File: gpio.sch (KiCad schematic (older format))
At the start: 3 parts, among them J1 DF40C-100DP-0.4V(51), J2 DF40C-100DP-0.4V(51), U1 LFE5U-85F-6BG381C

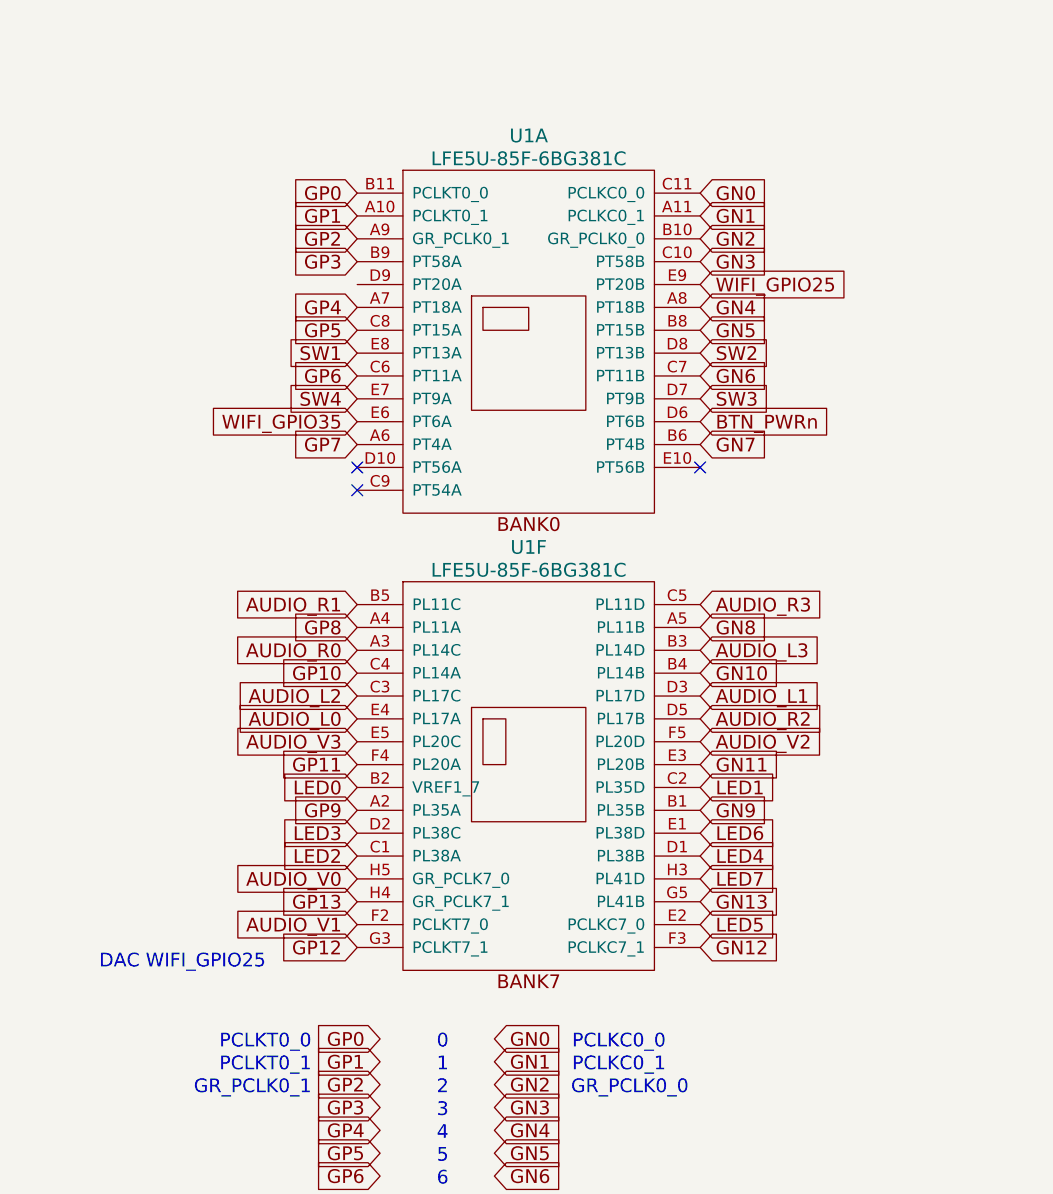
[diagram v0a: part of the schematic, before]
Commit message: Adding connectors
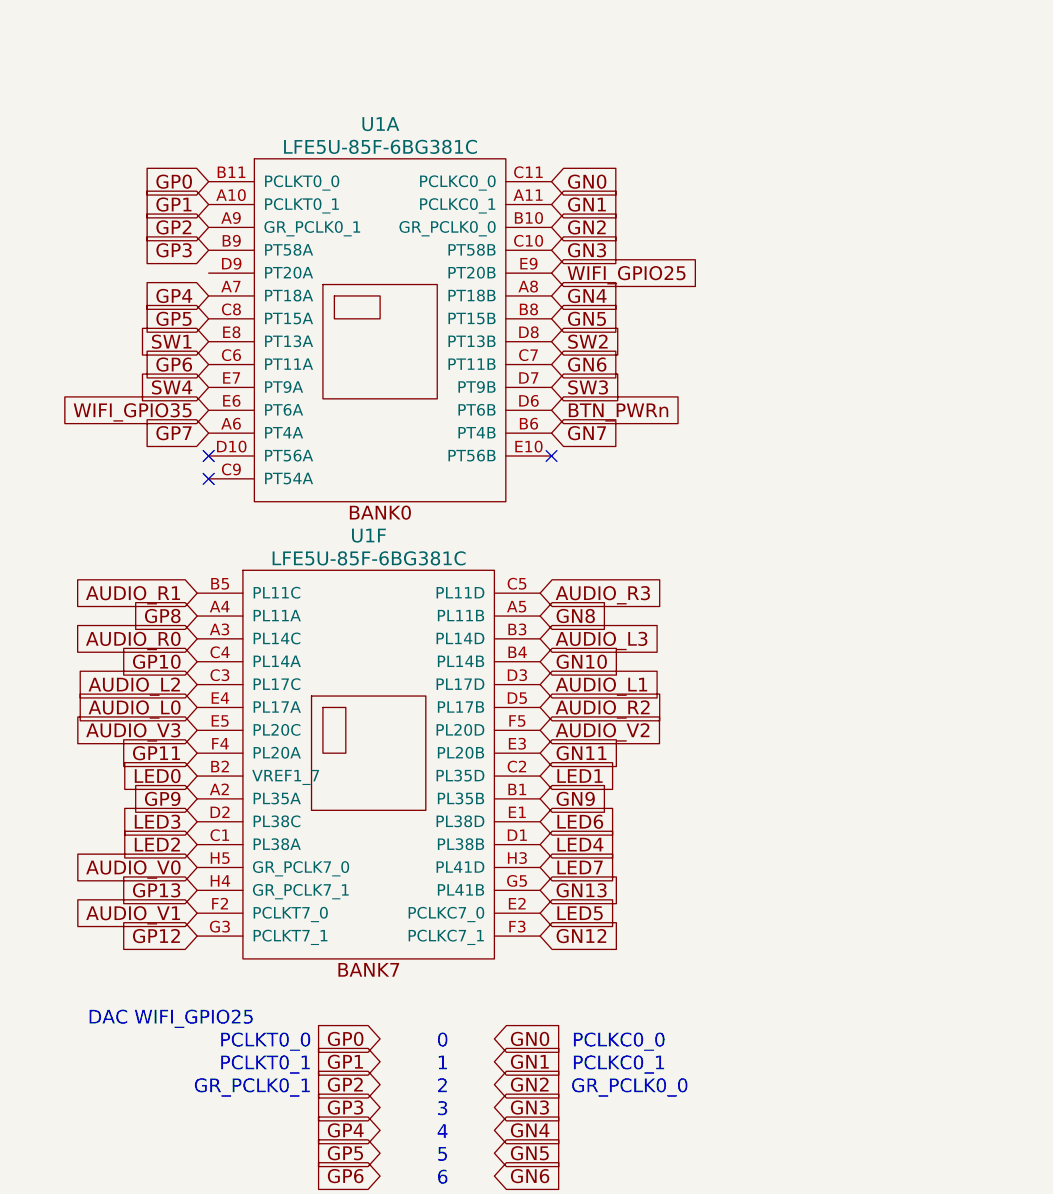
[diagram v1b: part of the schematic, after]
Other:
- moved on the sheet: U1A, U1F
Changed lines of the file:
@@
 Text GLabel 5350 6200 2    60   Input ~ 0
 GP27
-Text GLabel 3250 3950 2    60   Input ~ 0
+Text GLabel 2550 3900 2    60   Input ~ 0
 GN13
-Text GLabel 1750 3950 0    60   Input ~ 0
+Text GLabel 1050 3900 0    60   Input ~ 0
 GP13
-Text GLabel 1750 4150 0    60   Input ~ 0
+Text GLabel 1050 4100 0    60   Input ~ 0
 GP12
-Text GLabel 3250 4150 2    60   Input ~ 0
+Text GLabel 2550 4100 2    60   Input ~ 0
 GN12
-Text GLabel 3250 3350 2    60   Input ~ 0
+Text GLabel 2550 3300 2    60   Input ~ 0
 GN11
-Text GLabel 1750 3350 0    60   Input ~ 0
+Text GLabel 1050 3300 0    60   Input ~ 0
 GP11
-Text GLabel 3250 3550 2    60   Input ~ 0
+Text GLabel 2550 3500 2    60   Input ~ 0
 GN9
-Text GLabel 1750 3550 0    60   Input ~ 0
+Text GLabel 1050 3500 0    60   Input ~ 0
 GP9
-Text GLabel 3250 2950 2    60   Input ~ 0
+Text GLabel 2550 2900 2    60   Input ~ 0
 GN10
-Text GLabel 1750 2950 0    60   Input ~ 0
+Text GLabel 1050 2900 0    60   Input ~ 0
 GP10
-Text GLabel 3250 2750 2    60   Input ~ 0
+Text GLabel 2550 2700 2    60   Input ~ 0
 GN8
-Text GLabel 1750 2750 0    60   Input ~ 0
+Text GLabel 1050 2700 0    60   Input ~ 0
 GP8
-Text GLabel 3250 1950 2    60   Input ~ 0
+Text GLabel 2600 1900 2    60   Input ~ 0
 GN7
-Text GLabel 1750 1950 0    60   Input ~ 0
+Text GLabel 1100 1900 0    60   Input ~ 0
 GP7
-Text GLabel 3250 1650 2    60   Input ~ 0
+Text GLabel 2600 1600 2    60   Input ~ 0
 GN6
-Text GLabel 1750 1650 0    60   Input ~ 0
+Text GLabel 1100 1600 0    60   Input ~ 0
 GP6
-Text GLabel 3250 850  2    60   Input ~ 0
+Text GLabel 2600 800  2    60   Input ~ 0
 GN0
-Text GLabel 3250 950  2    60   Input ~ 0
+Text GLabel 2600 900  2    60   Input ~ 0
 GN1
-Text GLabel 3250 1050 2    60   Input ~ 0
+Text GLabel 2600 1000 2    60   Input ~ 0
 GN2
-Text GLabel 3250 1350 2    60   Input ~ 0
+Text GLabel 2600 1300 2    60   Input ~ 0
 GN4
-Text GLabel 1750 850  0    60   Input ~ 0
+Text GLabel 1100 800  0    60   Input ~ 0
 GP0
-Text GLabel 1750 950  0    60   Input ~ 0
+Text GLabel 1100 900  0    60   Input ~ 0
 GP1
-Text GLabel 1750 1050 0    60   Input ~ 0
+Text GLabel 1100 1000 0    60   Input ~ 0
 GP2
-Text GLabel 1750 1350 0    60   Input ~ 0
+Text GLabel 1100 1300 0    60   Input ~ 0
 GP4
-Text GLabel 1750 1450 0    60   Input ~ 0
+Text GLabel 1100 1400 0    60   Input ~ 0
 GP5
-Text GLabel 3250 1450 2    60   Input ~ 0
+Text GLabel 2600 1400 2    60   Input ~ 0
 GN5
-Text GLabel 3250 1150 2    60   Input ~ 0
+Text GLabel 2600 1100 2    60   Input ~ 0
 GN3
-Text GLabel 1750 1150 0    60   Input ~ 0
+Text GLabel 1100 1100 0    60   Input ~ 0
 GP3
-Text GLabel 1750 3150 0    60   Input ~ 0
+Text GLabel 1050 3100 0    60   Input ~ 0
 AUDIO_L0
-Text GLabel 3250 3050 2    60   Input ~ 0
+Text GLabel 2550 3000 2    60   Input ~ 0
 AUDIO_L1
-Text GLabel 1750 3050 0    60   Input ~ 0
+Text GLabel 1050 3000 0    60   Input ~ 0
 AUDIO_L2
-Text GLabel 3250 2850 2    60   Input ~ 0
+Text GLabel 2550 2800 2    60   Input ~ 0
 AUDIO_L3
-Text GLabel 1750 2850 0    60   Input ~ 0
+Text GLabel 1050 2800 0    60   Input ~ 0
 AUDIO_R0
-Text GLabel 1750 2650 0    60   Input ~ 0
+Text GLabel 1050 2600 0    60   Input ~ 0
 AUDIO_R1
-Text GLabel 3250 3150 2    60   Input ~ 0
+Text GLabel 2550 3100 2    60   Input ~ 0
 AUDIO_R2
-Text GLabel 3250 2650 2    60   Input ~ 0
+Text GLabel 2550 2600 2    60   Input ~ 0
 AUDIO_R3
-Text GLabel 1750 3450 0    60   Input ~ 0
+Text GLabel 1050 3400 0    60   Input ~ 0
 LED0
-Text GLabel 3250 4050 2    60   Input ~ 0
+Text GLabel 2550 4000 2    60   Input ~ 0
 LED5
-Text GLabel 1750 3750 0    60   Input ~ 0
+Text GLabel 1050 3700 0    60   Input ~ 0
 LED2
-Text GLabel 1750 3650 0    60   Input ~ 0
+Text GLabel 1050 3600 0    60   Input ~ 0
 LED3
-Text GLabel 3250 3750 2    60   Input ~ 0
+Text GLabel 2550 3700 2    60   Input ~ 0
 LED4
-Text GLabel 3250 3450 2    60   Input ~ 0
+Text GLabel 2550 3400 2    60   Input ~ 0
 LED1
-Text GLabel 3250 3650 2    60   Input ~ 0
+Text GLabel 2550 3600 2    60   Input ~ 0
 LED6
-Text GLabel 3250 3850 2    60   Input ~ 0
+Text GLabel 2550 3800 2    60   Input ~ 0
 LED7
 Text Notes 950  7550 0    60   ~ 0
 GPIO route only A/B pairs as those are differential bidirectional\ndon't route C/D pairs to GPIO as those can be differential input only\nBANK0,1 are single-ended (non-differential)
-Text GLabel 3250 1850 2    60   Input ~ 0
+Text GLabel 2600 1800 2    60   Input ~ 0
 BTN_PWRn
 Text Notes 950  7200 0    60   ~ 0
 GP,GN 14-21 differential bidirectional connected to BANK2,3 on "ram" sheet\nGP,GN 22-27 single-ended connected to BANK1 on "gpdi" sheet
-Text GLabel 1750 1550 0    60   Input ~ 0
+Text GLabel 1100 1500 0    60   Input ~ 0
 SW1
-Text GLabel 3250 1550 2    60   Input ~ 0
+Text GLabel 2600 1500 2    60   Input ~ 0
 SW2
-Text GLabel 3250 1750 2    60   Input ~ 0
+Text GLabel 2600 1700 2    60   Input ~ 0
 SW3
-Text GLabel 1750 1750 0    60   Input ~ 0
+Text GLabel 1100 1700 0    60   Input ~ 0
 SW4
-Text GLabel 1750 3250 0    60   Input ~ 0
+Text GLabel 1050 3200 0    60   Input ~ 0
 AUDIO_V3
-Text GLabel 3250 3250 2    60   Input ~ 0
+Text GLabel 2550 3200 2    60   Input ~ 0
 AUDIO_V2
-Text GLabel 1750 4050 0    60   Input ~ 0
+Text GLabel 1050 4000 0    60   Input ~ 0
 AUDIO_V1
-Text GLabel 1750 3850 0    60   Input ~ 0
+Text GLabel 1050 3800 0    60   Input ~ 0
 AUDIO_V0
 $Comp
 L lfe5bg381:LFE5UM-85F-6BG381C U1
 U 6 1 5A0783C9
-P 2500 3350
+P 1800 3300
 AR Path="/5A0783C9" Ref="U1"  Part="6"
 AR Path="/56AC389C/5A0783C9" Ref="U1"  Part="6"
-F 0 "U1" H 2500 4300 60  0000 C CNN
-F 1 "LFE5U-85F-6BG381C" H 2500 4200 60  0000 C CNN
-F 2 "lfe5bg381:BGA-381_pitch0.8mm_dia0.4mm" H 1450 4300 60  0001 C CNN
-F 3 "http://www.latticesemi.com/~/media/LatticeSemi/Documents/DataSheets/ECP5/FPGA-DS-02012.pdf" H 1450 4300 60  0001 C CNN
-F 4 "LFE5U-85F-6BG381C" H 2500 3350 60  0001 C CNN "MPN"
-	6    2500 3350
+F 0 "U1" H 1800 4250 60  0000 C CNN
+F 1 "LFE5U-85F-6BG381C" H 1800 4150 60  0000 C CNN
+F 2 "lfe5bg381:BGA-381_pitch0.8mm_dia0.4mm" H 750 4250 60  0001 C CNN
+F 3 "http://www.latticesemi.com/~/media/LatticeSemi/Documents/DataSheets/ECP5/FPGA-DS-02012.pdf" H 750 4250 60  0001 C CNN
+F 4 "LFE5U-85F-6BG381C" H 1800 3300 60  0001 C CNN "MPN"
+	6    1800 3300
 	1    0    0    -1
 $EndComp
@@
 L lfe5bg381:LFE5UM-85F-6BG381C U1
 U 1 1 5A0737C6
-P 2500 1550
+P 1850 1500
 AR Path="/5A0737C6" Ref="U1"  Part="1"
 AR Path="/56AC389C/5A0737C6" Ref="U1"  Part="1"
-F 0 "U1" H 2500 2500 60  0000 C CNN
-F 1 "LFE5U-85F-6BG381C" H 2500 2400 60  0000 C CNN
-F 2 "lfe5bg381:BGA-381_pitch0.8mm_dia0.4mm" H 1450 2500 60  0001 C CNN
-F 3 "http://www.latticesemi.com/~/media/LatticeSemi/Documents/DataSheets/ECP5/FPGA-DS-02012.pdf" H 1450 2500 60  0001 C CNN
-F 4 "LFE5U-85F-6BG381C" H 2500 1550 60  0001 C CNN "MPN"
-	1    2500 1550
+F 0 "U1" H 1850 2450 60  0000 C CNN
+F 1 "LFE5U-85F-6BG381C" H 1850 2350 60  0000 C CNN
+F 2 "lfe5bg381:BGA-381_pitch0.8mm_dia0.4mm" H 800 2450 60  0001 C CNN
+F 3 "http://www.latticesemi.com/~/media/LatticeSemi/Documents/DataSheets/ECP5/FPGA-DS-02012.pdf" H 800 2450 60  0001 C CNN
+F 4 "LFE5U-85F-6BG381C" H 1850 1500 60  0001 C CNN "MPN"
+	1    1850 1500
 	1    0    0    -1
 $EndComp
@@
 Text Notes 6300 7150 0    60   ~ 0
 STPS2L40AF
-NoConn ~ 1750 2050
-NoConn ~ 1750 2150
-NoConn ~ 3250 2050
+NoConn ~ 1100 2000
+NoConn ~ 1100 2100
+NoConn ~ 2600 2000
 Text Notes 1500 6100 2    60   ~ 0
 GR_PCLK7_1
@@
 Text Notes 3200 4800 2    60   ~ 0
 GR_PCLK0_0
-Text Notes 1350 4250 2    60   ~ 0
+Text Notes 1300 4500 2    60   ~ 0
 DAC WIFI_GPIO25
 Text Notes 1500 5900 2    60   ~ 0
@@
 Text Notes 950  6450 0    60   ~ 0
 J1 J2 PIN numbering 1-40 is for FEMALE 90° ANGLED header.\nFor MALE VERTICAL header, SWAP EVEN and ODD pin numbers.
-Text GLabel 3250 1250 2    60   Input ~ 0
+Text GLabel 2600 1200 2    60   Input ~ 0
 WIFI_GPIO25
-Text GLabel 1750 1850 0    60   Input ~ 0
+Text GLabel 1100 1800 0    60   Input ~ 0
 WIFI_GPIO35
 Text Notes 5700 7350 0    60   ~ 0
